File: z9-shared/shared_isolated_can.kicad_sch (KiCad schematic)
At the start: 9 parts

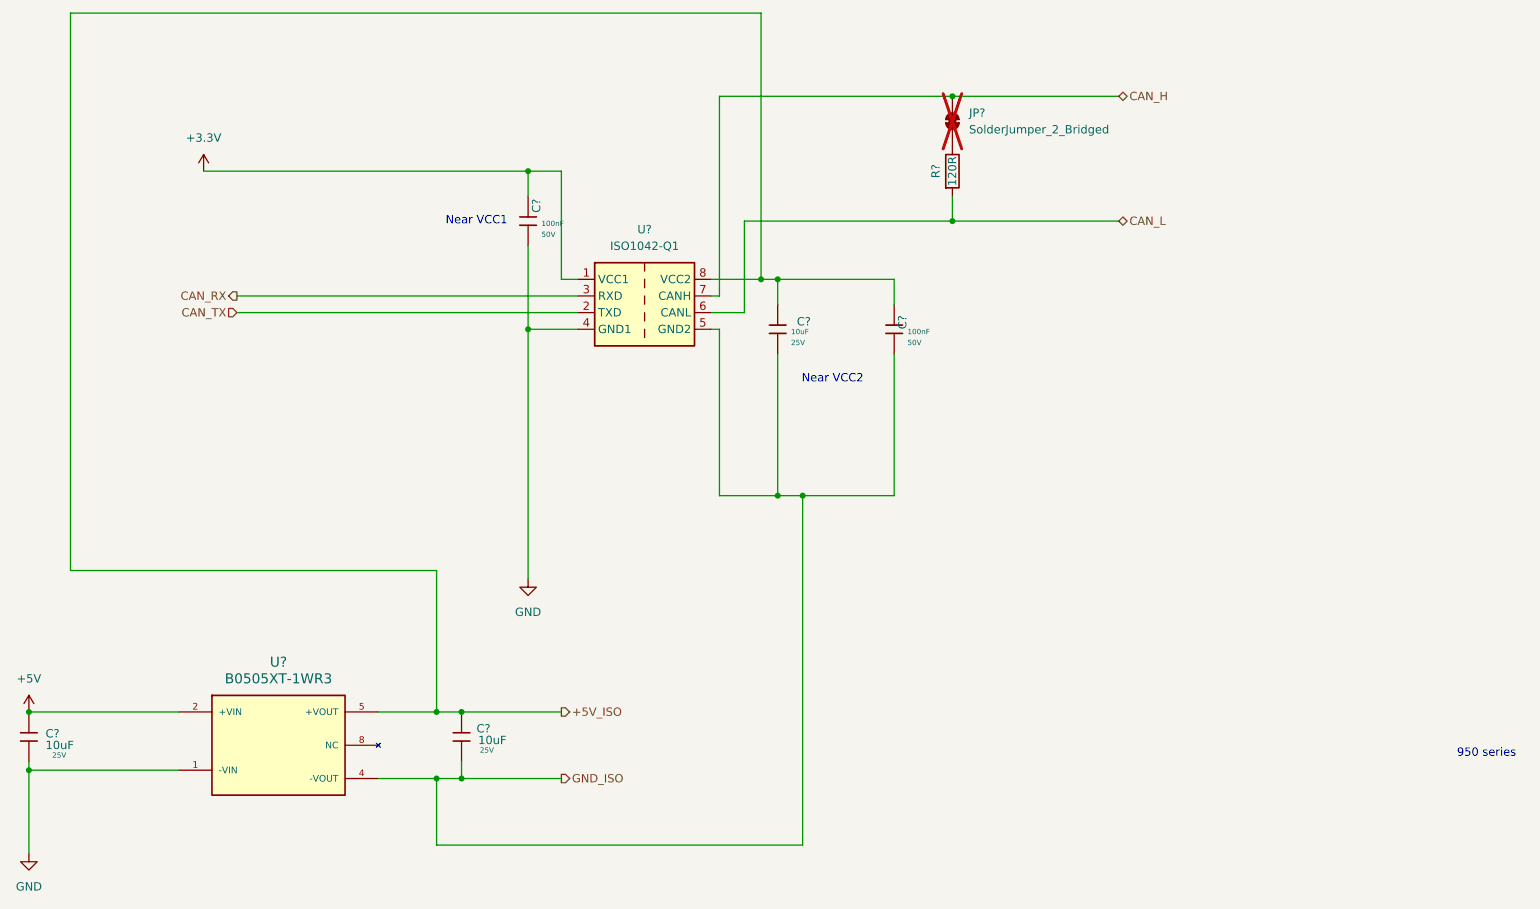
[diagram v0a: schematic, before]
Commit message: x
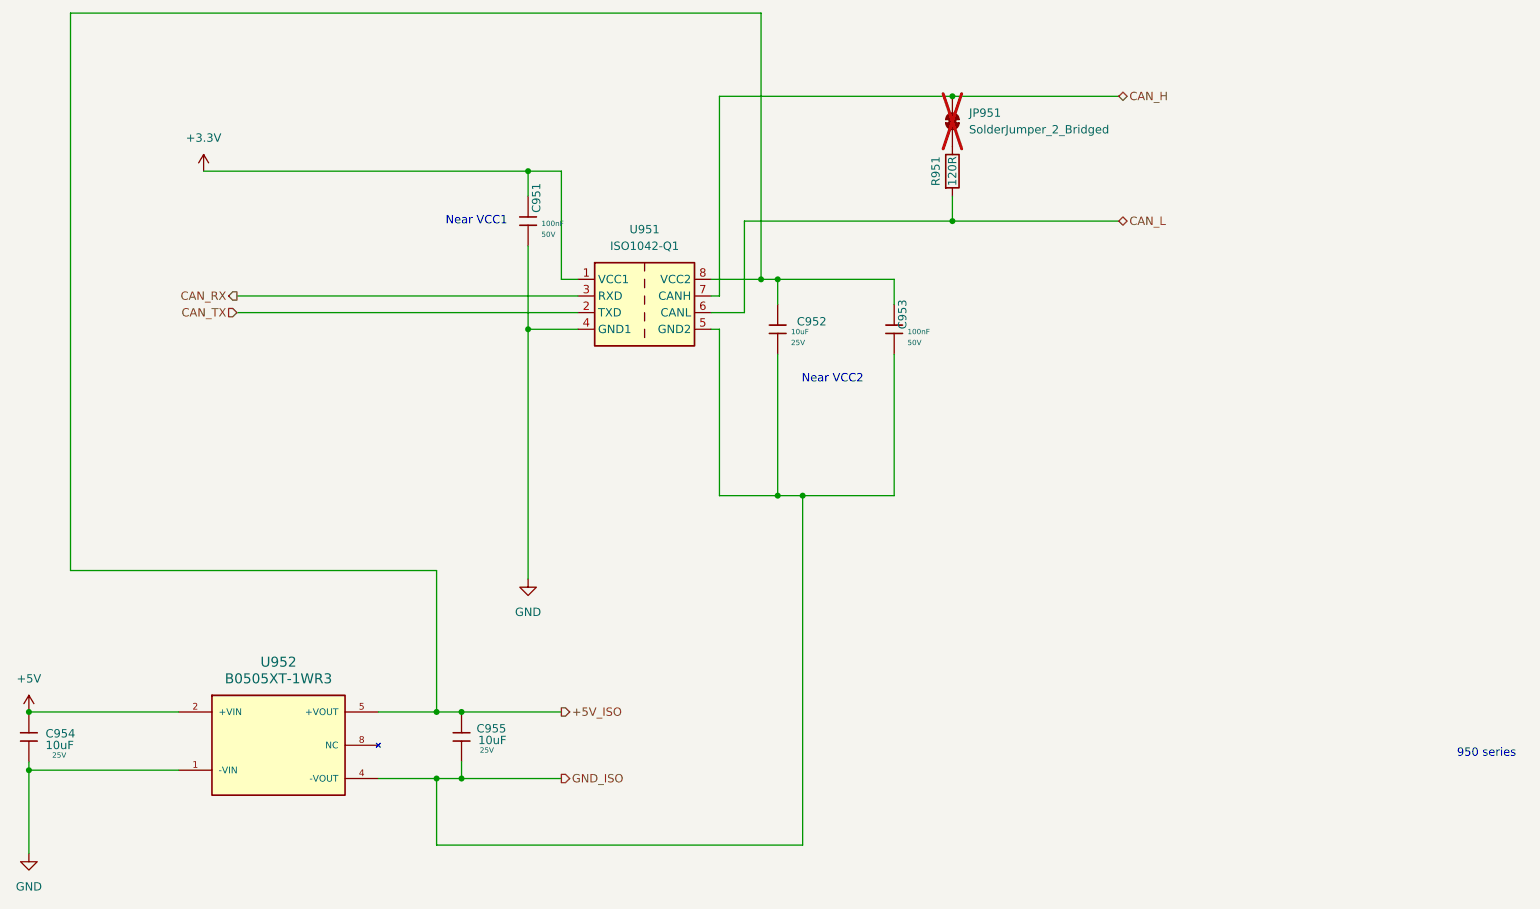
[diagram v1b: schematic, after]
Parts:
- gave numbers to parts that had none: 9
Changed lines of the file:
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@@
 		(dnp no)
 		(fields_autoplaced yes)
-		(property "Reference" "#PWR0117"
+		(property "Reference" "#PWR0111"
 			(at 128.27 142.24 0)
 			(effects
@@
 		(on_board yes)
 		(dnp no)
-		(property "Reference" "C?"
+		(property "Reference" "C953"
 			(at 185.42 97.79 90)
 			(effects
@@
 		(dnp no)
 		(fields_autoplaced yes)
-		(property "Reference" "#PWR0115"
+		(property "Reference" "#PWR0951"
 			(at 52.07 160.02 0)
 			(effects
@@
 		(on_board yes)
 		(dnp no)
-		(property "Reference" "R?"
+		(property "Reference" "R951"
 			(at 190.5 73.66 90)
 			(effects
@@
 		(on_board yes)
 		(dnp no)
-		(property "Reference" "C?"
+		(property "Reference" "C951"
 			(at 129.54 80.01 90)
 			(effects
@@
 		(on_board yes)
 		(dnp no)
-		(property "Reference" "C?"
+		(property "Reference" "C955"
 			(at 120.396 158.75 0)
 			(effects
@@
 		(on_board yes)
 		(dnp no)
-		(property "Reference" "C?"
+		(property "Reference" "C952"
 			(at 169.291 96.6216 0)
 			(effects
@@
 		(dnp no)
 		(fields_autoplaced yes)
-		(property "Reference" "#PWR0114"
+		(property "Reference" "#PWR0110"
 			(at 78.74 77.47 0)
 			(effects
@@
 		(on_board yes)
 		(dnp no)
-		(property "Reference" "C?"
+		(property "Reference" "C954"
 			(at 54.61 159.512 0)
 			(effects
@@
 		(dnp no)
 		(fields_autoplaced yes)
-		(property "Reference" "#PWR0116"
+		(property "Reference" "#PWR0952"
 			(at 52.07 184.15 0)
 			(effects
@@
 		(dnp no)
 		(fields_autoplaced yes)
-		(property "Reference" "U?"
+		(property "Reference" "U952"
 			(at 90.17 148.59 0)
 			(effects
@@
 		(dnp yes)
 		(fields_autoplaced yes)
-		(property "Reference" "JP?"
+		(property "Reference" "JP951"
 			(at 195.58 64.7699 90)
 			(effects
@@
 		(dnp no)
 		(fields_autoplaced yes)
-		(property "Reference" "U?"
+		(property "Reference" "U951"
 			(at 146.05 82.55 0)
 			(effects

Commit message: pre kicad update
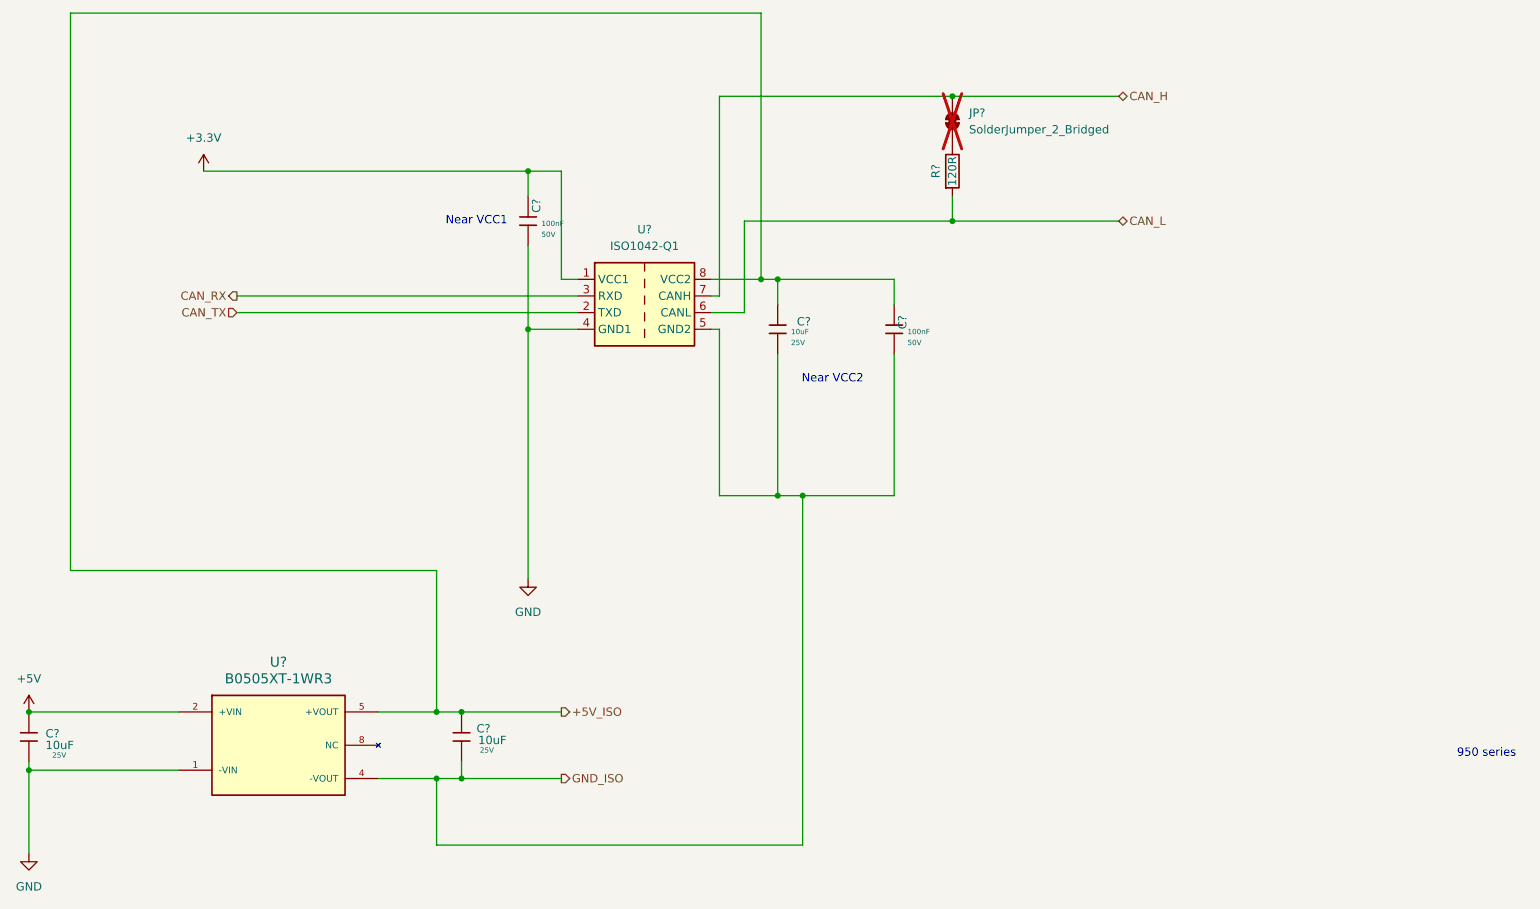
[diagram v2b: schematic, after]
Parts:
- renumbered C953 to C?, C951 to C?, C955 to C?, C952 to C?, C954 to C?, JP951 to JP?, R951 to R?, U952 to U?, U951 to U?
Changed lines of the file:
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@@
 		(dnp no)
 		(fields_autoplaced yes)
-		(property "Reference" "#PWR0111"
+		(property "Reference" "#PWR0117"
 			(at 128.27 142.24 0)
 			(effects
@@
 		(on_board yes)
 		(dnp no)
-		(property "Reference" "C953"
+		(property "Reference" "C?"
 			(at 185.42 97.79 90)
 			(effects
@@
 		(dnp no)
 		(fields_autoplaced yes)
-		(property "Reference" "#PWR0951"
+		(property "Reference" "#PWR0115"
 			(at 52.07 160.02 0)
 			(effects
@@
 		(on_board yes)
 		(dnp no)
-		(property "Reference" "R951"
+		(property "Reference" "R?"
 			(at 190.5 73.66 90)
 			(effects
@@
 		(on_board yes)
 		(dnp no)
-		(property "Reference" "C951"
+		(property "Reference" "C?"
 			(at 129.54 80.01 90)
 			(effects
@@
 		(on_board yes)
 		(dnp no)
-		(property "Reference" "C955"
+		(property "Reference" "C?"
 			(at 120.396 158.75 0)
 			(effects
@@
 		(on_board yes)
 		(dnp no)
-		(property "Reference" "C952"
+		(property "Reference" "C?"
 			(at 169.291 96.6216 0)
 			(effects
@@
 		(dnp no)
 		(fields_autoplaced yes)
-		(property "Reference" "#PWR0110"
+		(property "Reference" "#PWR0114"
 			(at 78.74 77.47 0)
 			(effects
@@
 		(on_board yes)
 		(dnp no)
-		(property "Reference" "C954"
+		(property "Reference" "C?"
 			(at 54.61 159.512 0)
 			(effects
@@
 		(dnp no)
 		(fields_autoplaced yes)
-		(property "Reference" "#PWR0952"
+		(property "Reference" "#PWR0116"
 			(at 52.07 184.15 0)
 			(effects
@@
 		(dnp no)
 		(fields_autoplaced yes)
-		(property "Reference" "U952"
+		(property "Reference" "U?"
 			(at 90.17 148.59 0)
 			(effects
@@
 		(dnp yes)
 		(fields_autoplaced yes)
-		(property "Reference" "JP951"
+		(property "Reference" "JP?"
 			(at 195.58 64.7699 90)
 			(effects
@@
 		(dnp no)
 		(fields_autoplaced yes)
-		(property "Reference" "U951"
+		(property "Reference" "U?"
 			(at 146.05 82.55 0)
 			(effects
